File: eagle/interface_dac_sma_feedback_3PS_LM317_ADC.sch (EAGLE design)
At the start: 43 parts, among them IC1 ISO1540, IC2 LT1352PA, IC3 LT1352PA, IC4 LM317MABDT, IC5 LM317MABDT, IC6 LM317MABDT, Q1 TIP122V, Q2 TIP122V, Q3 TIP122V, X1 BU-SMA-V

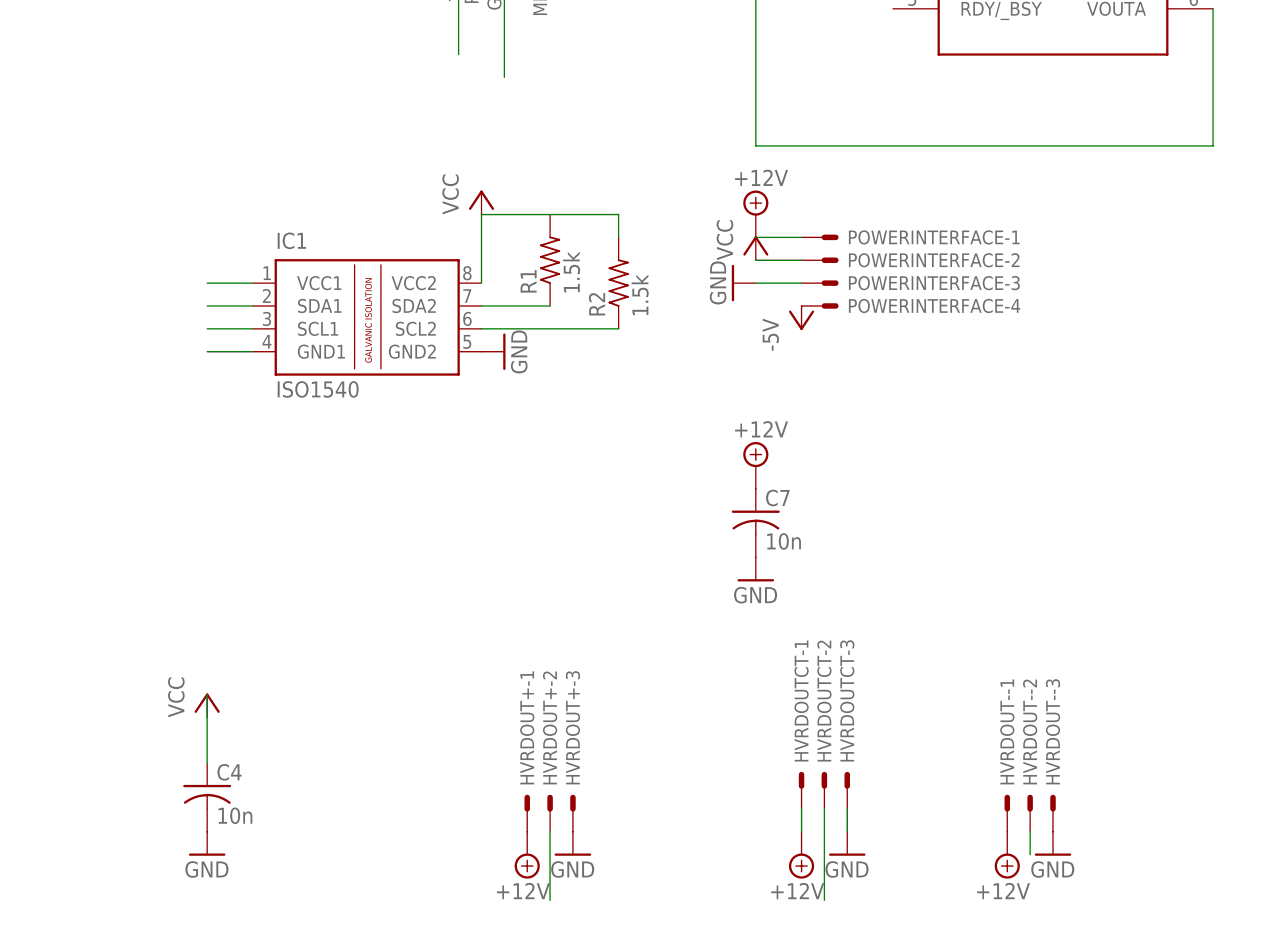
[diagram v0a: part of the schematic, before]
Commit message: Readbacks
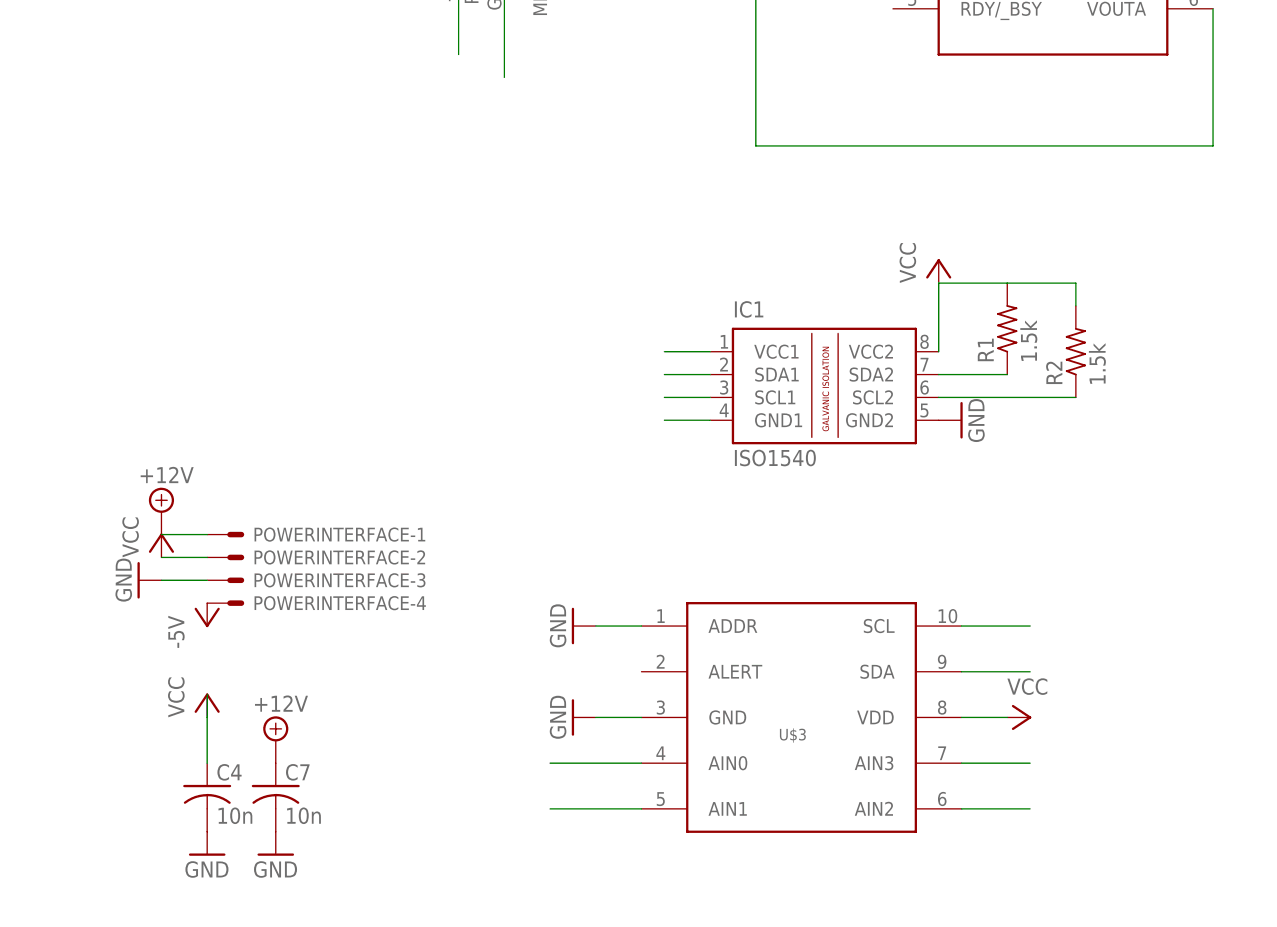
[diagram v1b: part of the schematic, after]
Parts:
- removed HVRDOUT+, HVRDOUT-, HVRDOUTCT: (no value), con-molex:KK-156-3
- added U$3: ADS1015DIL, texas:ADS1015DIL
- C1: device rcl:C-US050-050X075 -> rcl:C-US050-024X044
- C4: device resistor:C-US075-063X106 -> resistor:C-US050-024X044
- C7: device resistor:C-US050-050X075 -> resistor:C-US050-024X044
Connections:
- removed net N$27: IC3A.-IN, R13.2, R9.1
- removed net N$6: FDBKHV-2.S, HVRDOUTCT-2.S, IC2B.-IN, R4.1
- removed net N$8: FDBKHV-1.S, HVRDOUT+-2.S, IC2A.-IN, R3.1
- new net RDBK1: FDBKHV-1.S, IC2A.-IN, R3.1, U$3.AIN0
- new net RDBK2: FDBKHV-2.S, IC2B.-IN, R4.1, U$3.AIN1
- new net RDBK3: IC3A.-IN, R13.2, R9.1, U$3.AIN2
- new net RDBK4: C2.1, U$1.P$1, U$3.AIN3
- net +12V: no longer HVRDOUT+-1.S, HVRDOUT--1.S, HVRDOUTCT-1.S
- net GND: now also U$3.ADDR, U$3.GND; no longer HVRDOUT+-3.S, HVRDOUT--3.S, HVRDOUTCT-3.S
- net N$14: no longer HVRDOUT--2.S
- net N$2: no longer C2.1, U$1.P$1
- net SCL_OUT: now also U$3.SCL
- net SDA_OUT: now also U$3.SDA
- net VCC: now also U$3.VDD
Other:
- moved on the sheet: C7, IC1, POWERINTERFACE-1, POWERINTERFACE-2, POWERINTERFACE-3, POWERINTERFACE-4, R1, R2
